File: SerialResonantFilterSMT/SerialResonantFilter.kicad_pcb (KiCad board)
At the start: 2 copper layers, 31.8 x 106.7 mm, 44 parts, among them J1 OUT, J2 INP, J3 INP, J4 OUT, J5 INP, J6 OUT, J7 INP, J8 OUT

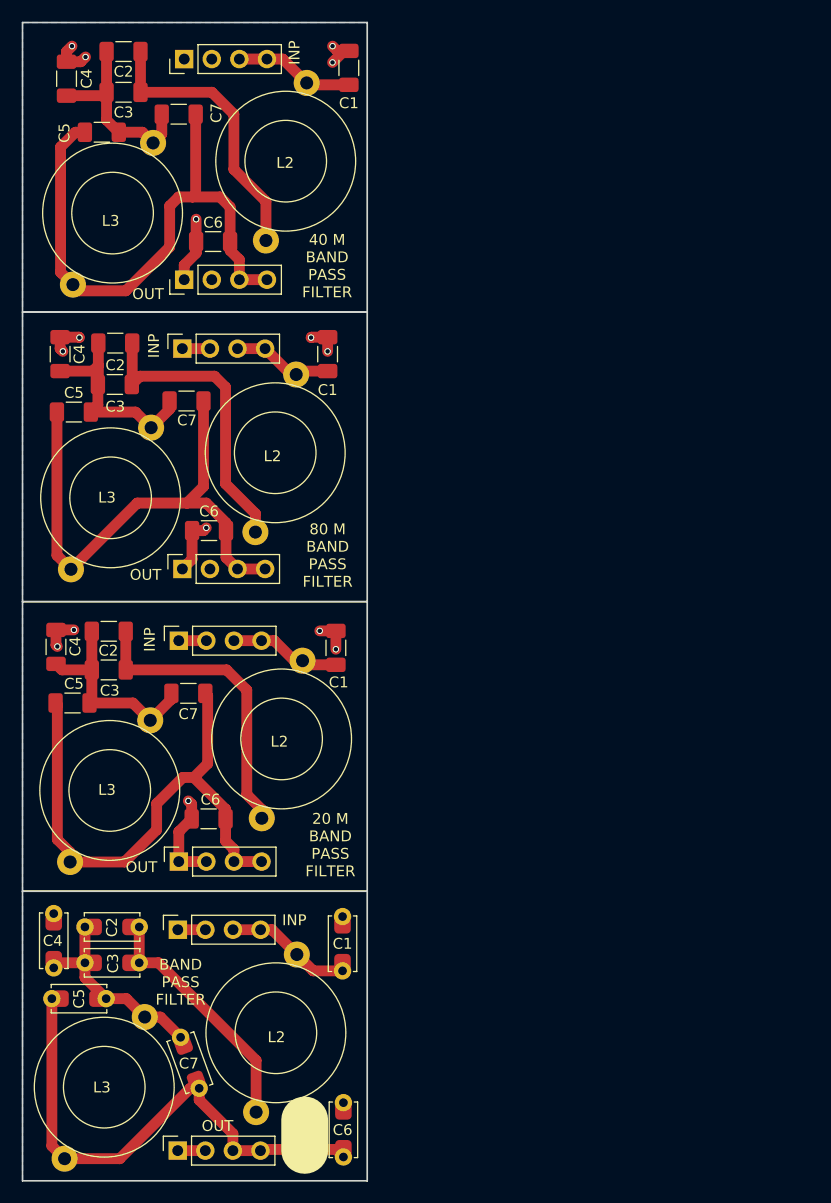
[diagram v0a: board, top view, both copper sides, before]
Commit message: Made six panel version of SerialResonantFilterSMT
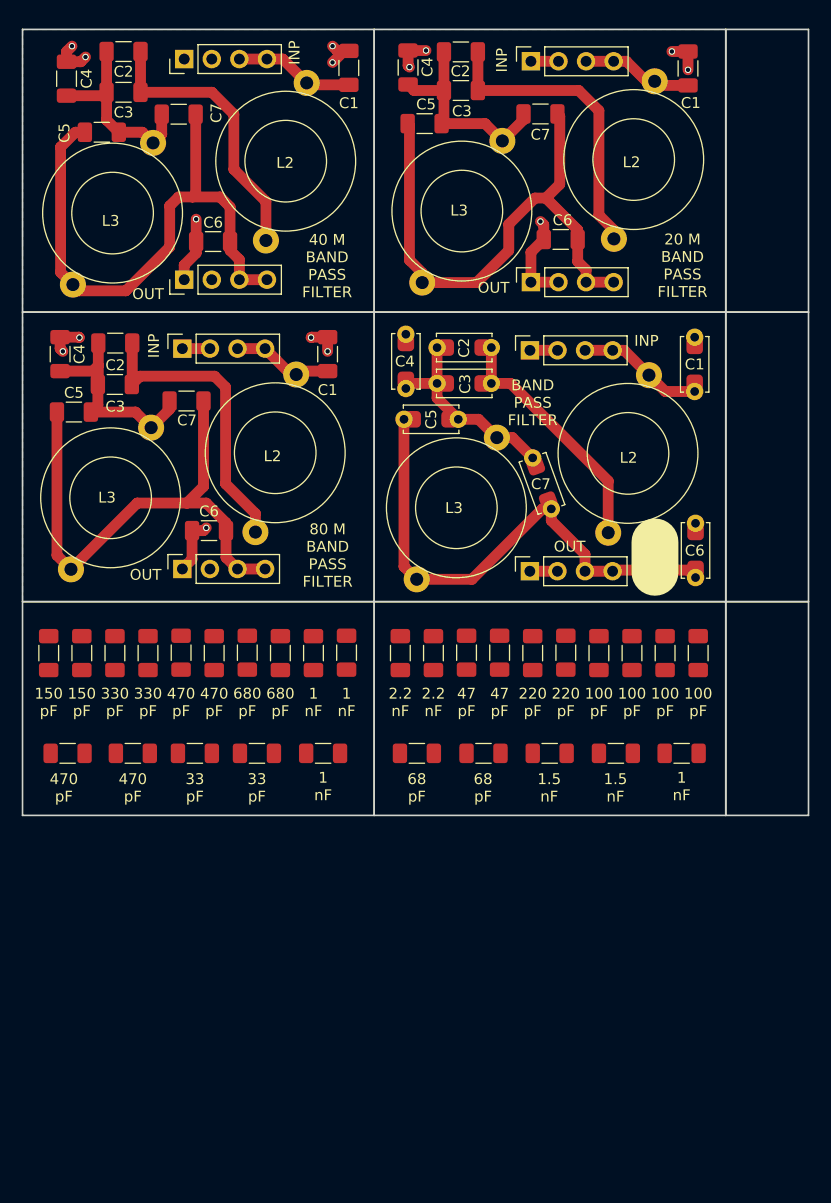
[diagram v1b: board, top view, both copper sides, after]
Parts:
- added C29: 330 pF, Capacitor_SMD:C_1206_3216Metric_Pad1.33x1.80mm_HandSolder, F.Cu at (127.1, 97.4)
- added C30: 150 pF, Capacitor_SMD:C_1206_3216Metric_Pad1.33x1.80mm_HandSolder, F.Cu at (118.0, 97.4)
- added C31: 470 pF, Capacitor_SMD:C_1206_3216Metric_Pad1.33x1.80mm_HandSolder, F.Cu at (130.2, 97.4)
- added C32: 330 pF, Capacitor_SMD:C_1206_3216Metric_Pad1.33x1.80mm_HandSolder, F.Cu at (124.1, 97.4)
- added C33: 150 pF, Capacitor_SMD:C_1206_3216Metric_Pad1.33x1.80mm_HandSolder, F.Cu at (121.0, 97.4)
- added C34: 470 pF, Capacitor_SMD:C_1206_3216Metric_Pad1.33x1.80mm_HandSolder, F.Cu at (133.2, 97.4)
- added C35: 680 pF, Capacitor_SMD:C_1206_3216Metric_Pad1.33x1.80mm_HandSolder, F.Cu at (139.3, 97.4)
- added C36: 2200 pF, Capacitor_SMD:C_1206_3216Metric_Pad1.33x1.80mm_HandSolder, F.Cu at (150.4, 97.4)
- added C37: 1000 pF, Capacitor_SMD:C_1206_3216Metric_Pad1.33x1.80mm_HandSolder, F.Cu at (142.4, 97.4)
- added C38: 680 pF, Capacitor_SMD:C_1206_3216Metric_Pad1.33x1.80mm_HandSolder, F.Cu at (136.3, 97.4)
- added C39: 2200 pF, Capacitor_SMD:C_1206_3216Metric_Pad1.33x1.80mm_HandSolder, F.Cu at (153.4, 97.4)
- added C40: 1000 pF, Capacitor_SMD:C_1206_3216Metric_Pad1.33x1.80mm_HandSolder, F.Cu at (145.4, 97.4)
- added C41: 100 pF, Capacitor_SMD:C_1206_3216Metric_Pad1.33x1.80mm_HandSolder, F.Cu at (168.7, 97.4)
- added C42: 47 pF, Capacitor_SMD:C_1206_3216Metric_Pad1.33x1.80mm_HandSolder, F.Cu at (159.5, 97.4)
- added C43: 220 pF, Capacitor_SMD:C_1206_3216Metric_Pad1.33x1.80mm_HandSolder, F.Cu at (165.6, 97.4)
- added C44: 100 pF, Capacitor_SMD:C_1206_3216Metric_Pad1.33x1.80mm_HandSolder, F.Cu at (177.8, 97.4)
- added C45: 47 pF, Capacitor_SMD:C_1206_3216Metric_Pad1.33x1.80mm_HandSolder, F.Cu at (156.5, 97.4)
- added C46: 100 pF, Capacitor_SMD:C_1206_3216Metric_Pad1.33x1.80mm_HandSolder, F.Cu at (174.8, 97.4)
- added C47: 100 pF, Capacitor_SMD:C_1206_3216Metric_Pad1.33x1.80mm_HandSolder, F.Cu at (171.7, 97.4)
- added C48: 220 pF, Capacitor_SMD:C_1206_3216Metric_Pad1.33x1.80mm_HandSolder, F.Cu at (162.6, 97.4)
- added C49: 33 pF, Capacitor_SMD:C_1206_3216Metric_Pad1.33x1.80mm_HandSolder, F.Cu at (131.4, 106.7)
- added C50: 33 pF, Capacitor_SMD:C_1206_3216Metric_Pad1.33x1.80mm_HandSolder, F.Cu at (137.2, 106.7)
- added C51: 470 pF, Capacitor_SMD:C_1206_3216Metric_Pad1.33x1.80mm_HandSolder, F.Cu at (119.7, 106.7)
- added C52: 470 pF, Capacitor_SMD:C_1206_3216Metric_Pad1.33x1.80mm_HandSolder, F.Cu at (125.7, 106.7)
- added C53: 68 pF, Capacitor_SMD:C_1206_3216Metric_Pad1.33x1.80mm_HandSolder, F.Cu at (151.9, 106.7)
- added C54: 68 pF, Capacitor_SMD:C_1206_3216Metric_Pad1.33x1.80mm_HandSolder, F.Cu at (158.0, 106.7)
- added C55: 1500 pF, Capacitor_SMD:C_1206_3216Metric_Pad1.33x1.80mm_HandSolder, F.Cu at (170.2, 106.7)
- added C56: 1500 pF, Capacitor_SMD:C_1206_3216Metric_Pad1.33x1.80mm_HandSolder, F.Cu at (164.1, 106.7)
- added C57: 1000 pF, Capacitor_SMD:C_1206_3216Metric_Pad1.33x1.80mm_HandSolder, F.Cu at (176.3, 106.7)
- added C58: 1000 pF, Capacitor_SMD:C_1206_3216Metric_Pad1.33x1.80mm_HandSolder, F.Cu at (143.3, 106.7)
- C1: value C1 -> 330 pF
- C10: value C2 -> 470 pF
- C11: value C4 -> 470 pF
- C13: value C5 -> 150 pF
- C14: value C6 -> 470 pF
- C15: value C1 -> 680 pF
- C17: value C2 -> 2200 pF
- C18: value C4 -> 2200 pF
- C2: value C2 -> 1000 pF
- C20: value C5 -> 680 pF
- C21: value C6 -> 2200 pF
- C4: value C4 -> 1000 pF
- C5: value C5 -> 330 pF
- C6: value C6 -> 1000 pF
- C8: value C1 -> 150 pF
- L1: value L2 -> 0.39 uH
- L2: value L2 -> 0.77 uH
- L3: value L3 -> 0.36 uH
- L4: value L3 -> 0.18 uH
- L5: value L2 -> 1.45 uH
- L6: value L3 -> 0.68 uH
- moved C10 62.4 mm to (155.9, 42.1)
- moved C22 62.4 mm to (177.5, 68.4)
- moved C25 62.4 mm to (150.9, 68.1)
- moved C9 62.4 mm to (155.9, 45.6)
- moved J7 62.4 mm to (162.3, 69.6)
- moved L7 62.4 mm to (173.9, 69.4)
- moved C14 62.4 mm to (165.1, 59.3)
- moved J3 62.4 mm to (162.4, 42.9)
- moved J4 62.4 mm to (162.4, 63.3)
- moved J8 62.4 mm to (162.3, 89.9)
- moved L1 62.4 mm to (174.4, 42.3)
- moved C12 62.4 mm to (163.3, 47.8)
- moved C23 62.4 mm to (158.8, 72.6)
- moved C24 62.4 mm to (158.8, 69.3)
- moved C26 62.4 mm to (162.6, 79.5)
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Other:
- board size 31.8 x 106.7 mm -> 72.4 x 72.4 mm
- board text added: "1 nF"
- board text added: "1.5 nF"
- board text added: "100 pF"
- board text added: "150 pF"
- board text added: "2.2 nF"
- board text added: "220 pF"
- board text added: "33 pF"
- board text added: "330 pF"
- board text added: "47 pF"
- board text added: "470 pF"
- board text added: "68 pF"
- board text added: "680 pF"
- board text added: "C1, C5: 150 PF C2, C4, C6: 470 PF C3, C7: NC 1206 NP0/C0G 100 V MIN"
- board text added: "C1, C5: 330 PF C2, C4, C6: 1000 PF C3, C7: NC 1206 NP0/C0G 100 V MIN"
- board text added: "C1, C5: 680 PF C2, C4, C6: 2200 PF C3, C7: NC 1206 NP0/C0G 100 V MIN"
- board text removed: "C1, C5: 150 PF C2, C4, C6: 470 PF C3, C7: NC 1206 NP0/C0G"
- board text removed: "C1, C5: 330 PF C2, C4, C6: 1000 PF C3, C7: NC 1206 NP0/C0G"
- board text removed: "C1, C5: 680 PF C2, C4, C6: 2200 PF C3, C7: NC 1206 NP0/C0G"
